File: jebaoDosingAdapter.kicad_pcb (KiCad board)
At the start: 2 copper layers, 33.8 x 25.2 mm, 5 parts, among them J1 Conn_01x05_Male, J2 Conn_01x02_Male, J3 6P6C, U1 ULN2803A

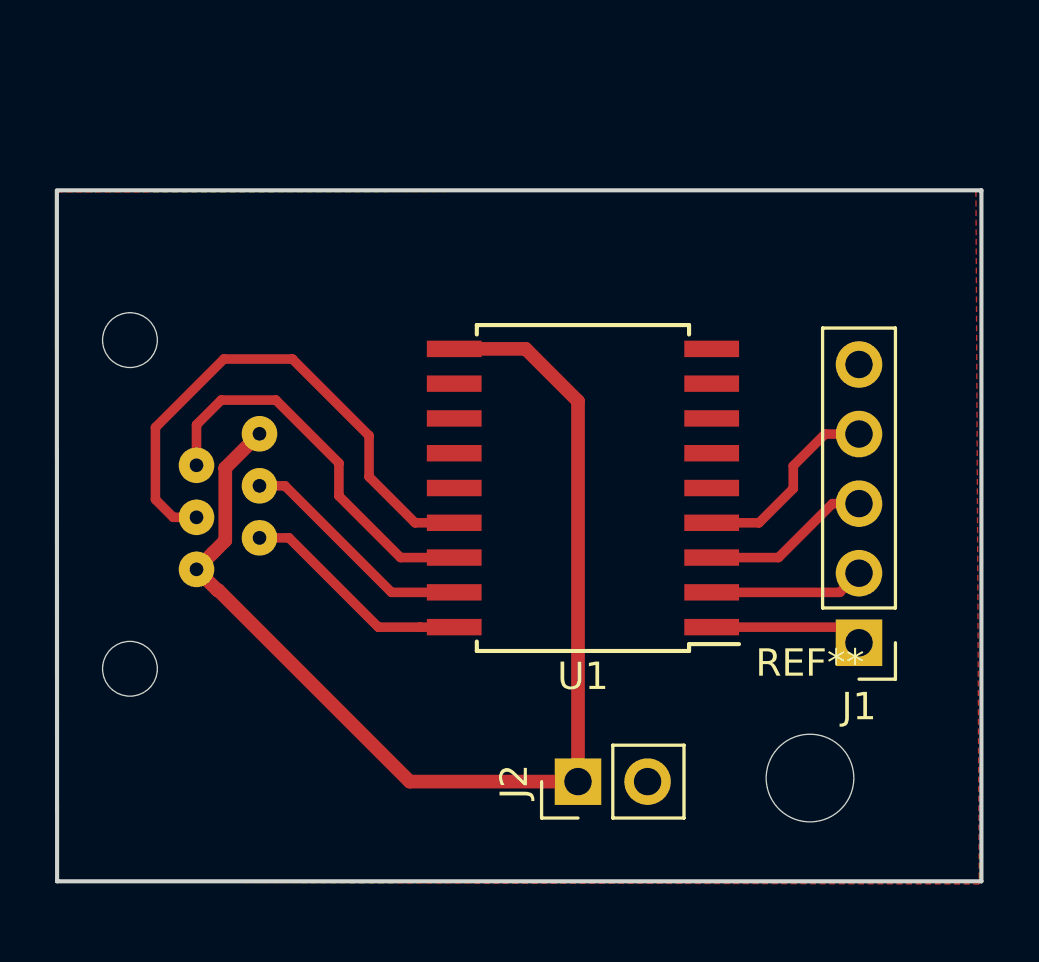
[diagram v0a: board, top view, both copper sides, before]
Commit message: Add images and updated gerbers
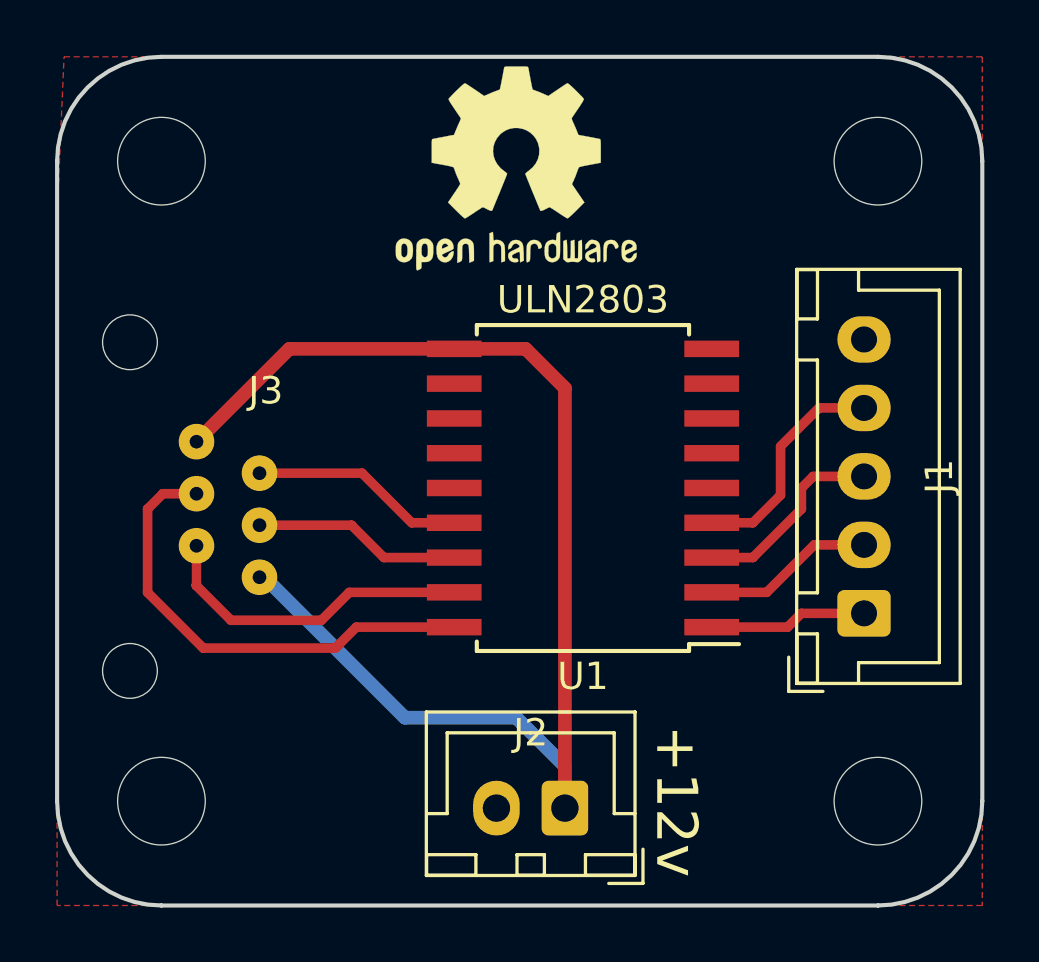
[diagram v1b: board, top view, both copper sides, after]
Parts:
- removed the REF** at (105.0, 82.0)
- added G***: LOGO, ml_logo:ML_Logo, B.Cu at (99.3, 73.9)
- added H1: MountingHole, MountingHole:MountingHole_3.2mm_M3, F.Cu at (107.4, 59.4)
- added H2: MountingHole, MountingHole:MountingHole_3.2mm_M3, F.Cu at (107.4, 82.8)
- added H3: MountingHole, MountingHole:MountingHole_3.2mm_M3, F.Cu at (81.3, 59.4)
- added H4: MountingHole, MountingHole:MountingHole_3.2mm_M3, F.Cu at (81.3, 82.8)
- added REF**: OSHW-Logo2_9.8x8mm_SilkScreen, Symbol:OSHW-Logo2_9.8x8mm_SilkScreen, F.Cu at (94.2, 59.7)
- J1: footprint Connector_PinHeader_2.54mm:PinHeader_1x05_P2.54mm_Vertical -> Connector_JST:JST_XH_B05B-XH-A_1x05_P2.50mm_Vertical
- J2: footprint Connector_PinHeader_2.54mm:PinHeader_1x02_P2.54mm_Vertical -> Connector_JST:JST_XH_B02B-XH-A_1x02_P2.50mm_Vertical
- J3: moved to F.Cu
- U1: value ULN2803A -> ULN2803
- moved J3 10.9 mm to (87.6, 66.5)
- moved J1 1.09 mm to (106.9, 75.9), turned to 90 degrees
- moved J2 1.08 mm to (96.0, 83.1), turned to 180 degrees
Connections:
- J3 pad 2: Net-(J3-Pad2) -> /O2
- J3 pad 3: Net-(J3-Pad3) -> /O3
- J3 pad 4: Net-(J3-Pad4) -> /O1
- J3 pad 5: Net-(J3-Pad5) -> /O4
- U1 pad 15: Net-(J3-Pad4) -> /O4
- U1 pad 16: Net-(J3-Pad2) -> /O3
- U1 pad 17: Net-(J3-Pad3) -> /O2
- U1 pad 18: Net-(J3-Pad5) -> /O1
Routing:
- net Net-(J3-Pad4): track 19.7 -> 0.00 mm
- net /O1: track 0.00 -> 17.4 mm
- net Net-(J3-Pad2): track 14.3 -> 0.00 mm
- net /O2: track 0.00 -> 11.8 mm
- net Net-(J3-Pad3): track 8.72 -> 0.00 mm
- net Net-(J3-Pad5): track 8.46 -> 0.00 mm
- net /O4: track 0.00 -> 7.86 mm
- net /O3: track 0.00 -> 7.60 mm
- net +12V: track 43.0 -> 47.1 mm
- net Net-(J1-Pad4): track 7.21 -> 8.34 mm
- net Net-(J1-Pad3): track 6.20 -> 7.24 mm
- net Net-(J1-Pad2): track 5.67 -> 6.28 mm
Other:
- board size 33.8 x 25.2 mm -> 33.8 x 31 mm
- board text added: "+12v"
- board text added: "Jebao doser adapter github.com/ranthalion/ jebaoDosingAdapter"
